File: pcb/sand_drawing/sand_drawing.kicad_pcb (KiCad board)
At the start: 2 copper layers, 67 x 80.4 mm, 38 parts, among them J0 12V GND, J1 Stepper1, J2 Stepper2, J3 Opto 1, J4 Opto 2, J5 UART, SW1 EN, SW2 IO0, U2 AMS1117-3.3, U3 ESP32-WROOM-32D

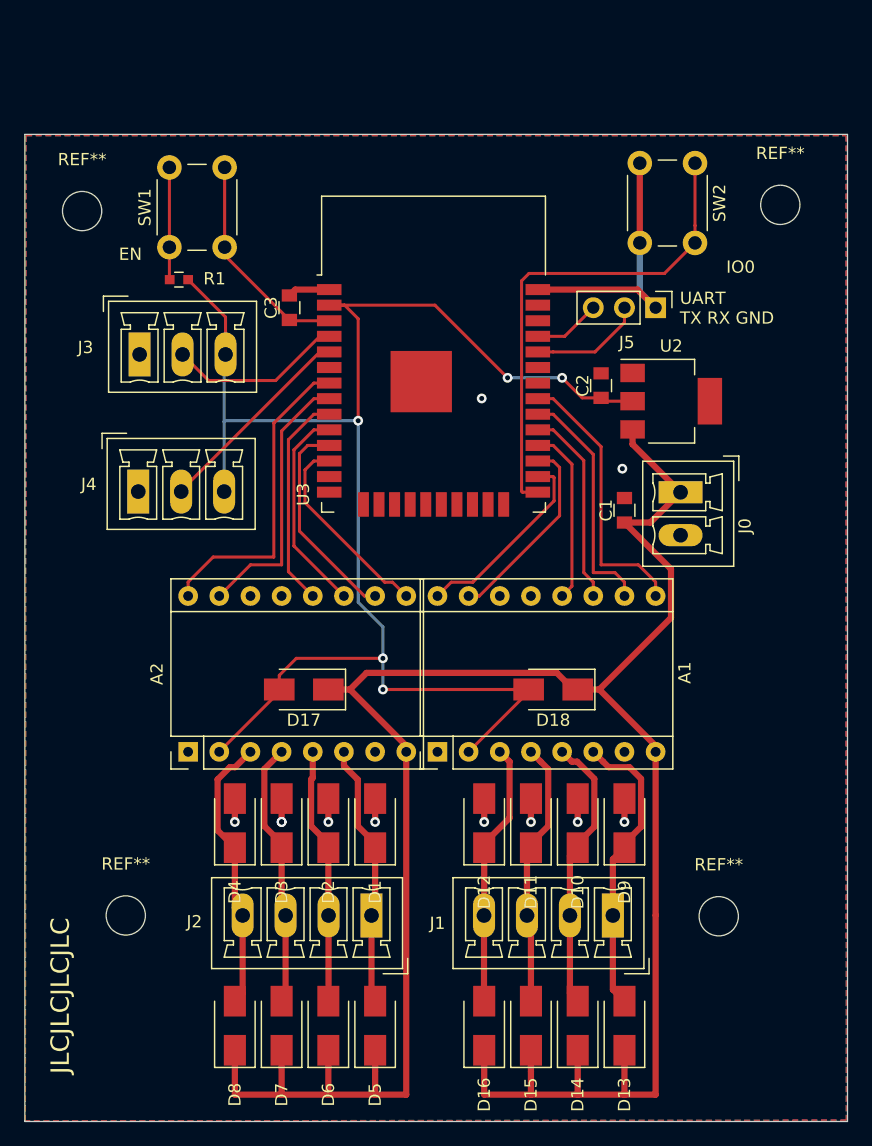
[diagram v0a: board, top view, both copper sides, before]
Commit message: Final tweaks. v1.0 PCB done!
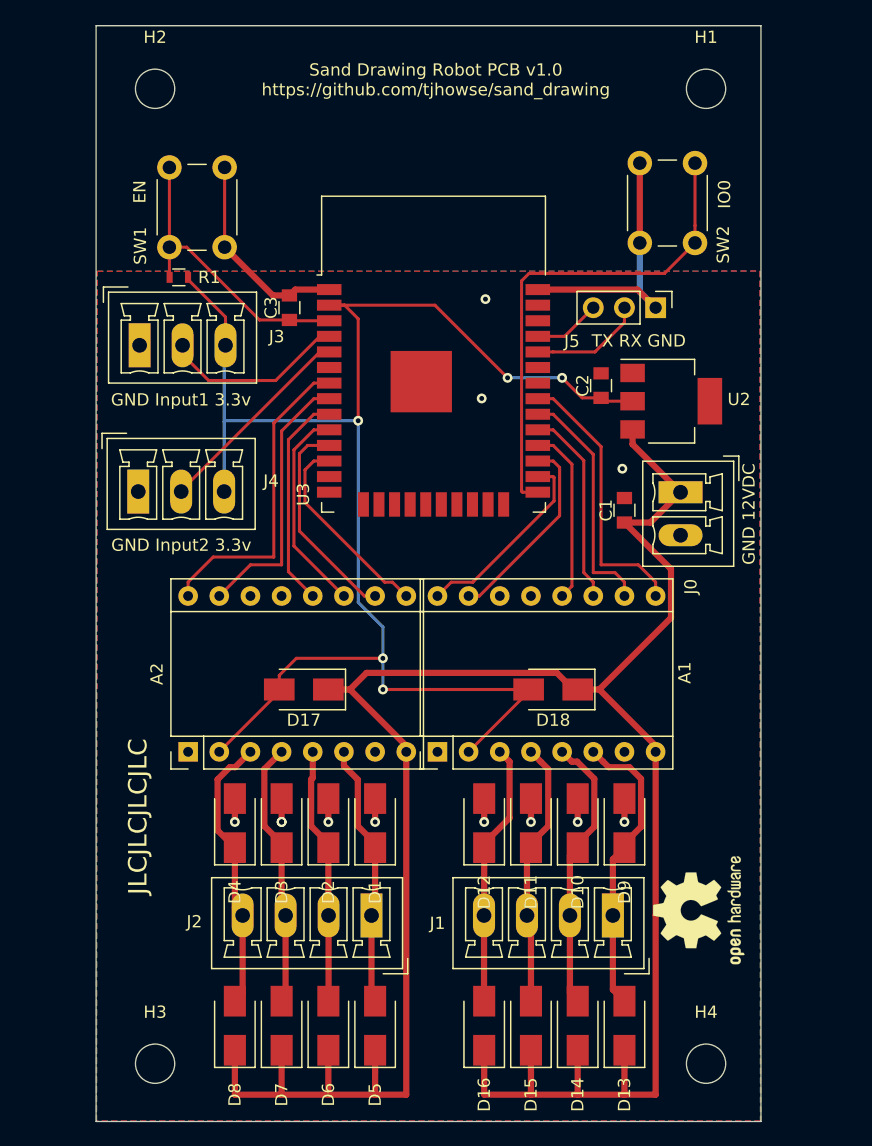
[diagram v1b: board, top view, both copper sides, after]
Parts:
- removed REF** (x4): MountingHole_3.2mm_M3, Mounting_Holes:MountingHole_3.2mm_M3
- added H1: MountingHole, Mounting_Holes:MountingHole_3.2mm_M3, F.Cu at (146.3, 80.0)
- added H2: MountingHole, Mounting_Holes:MountingHole_3.2mm_M3, F.Cu at (101.5, 80.0)
- added H3: MountingHole, Mounting_Holes:MountingHole_3.2mm_M3, F.Cu at (101.5, 159.4)
- added H4: MountingHole, Mounting_Holes:MountingHole_3.2mm_M3, F.Cu at (146.3, 159.4)
- added LOGO1: OSHW-Logo2_9.8x8mm_SilkScreen, Symbols:OSHW-Logo2_9.8x8mm_SilkScreen, F.Cu at (145.8, 146.9)
- C3: value 10µF/25V -> 100pF/50V
- R1: footprint Capacitors_SMD:C_0603 -> Resistors_SMD:R_0603
- moved J3 0.75 mm to (100.2, 100.9)
- moved R1 0.19 mm to (103.4, 95.3)
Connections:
- R1 pad 2: Net-(R1-Pad2) -> Net-(C3-Pad1)
- SW1 pad 1: Net-(R1-Pad2) -> Net-(C3-Pad1)
- SW1 pad 2: Net-(C3-Pad1) -> GND
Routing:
- net GND: track 41.2 -> 55.3 mm, vias 11 -> 12
- net Net-(R1-Pad2): track 9.15 -> 0.00 mm
- net Net-(C3-Pad1): track 17.5 -> 24.3 mm
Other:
- board size 67 x 80.4 mm -> 54.2 x 89.3 mm
- board text added: "GND 12VDC"
- board text added: "GND Input1 3.3v"
- board text added: "GND Input2 3.3v"
- board text added: "Love to Michelle, Alex and Sam"
- board text added: "Sand Drawing Robot PCB v1.0 https://github.com/tjhowse/sand_drawing"
- board text added: "TX RX GND"
- board text removed: "UART TX RX GND"
